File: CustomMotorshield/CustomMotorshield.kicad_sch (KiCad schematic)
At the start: 7 parts, among them J1 Conn_01x20, J2 Conn_01x20

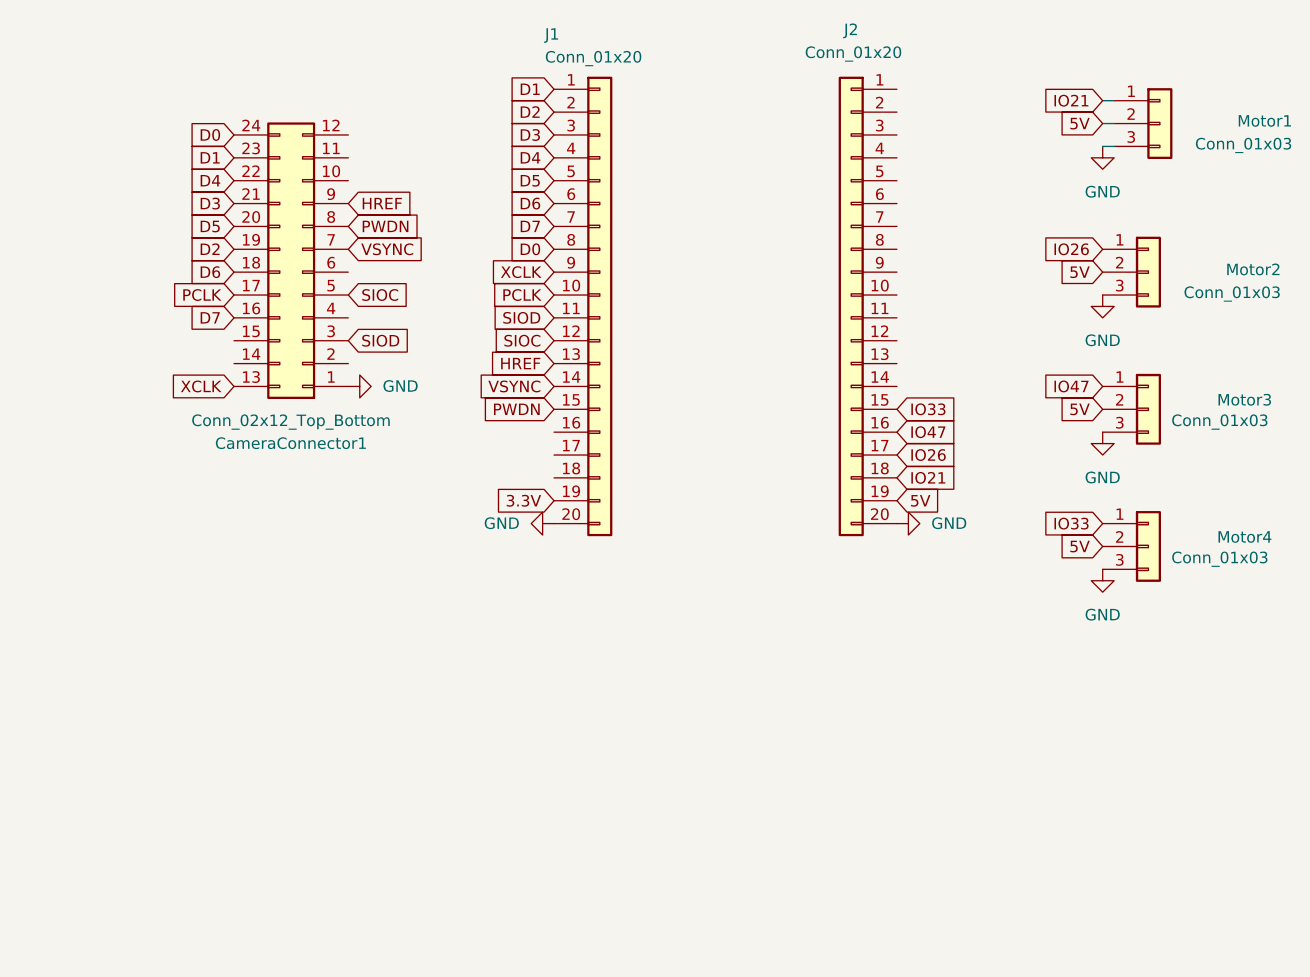
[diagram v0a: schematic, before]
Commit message: Updated PCB !
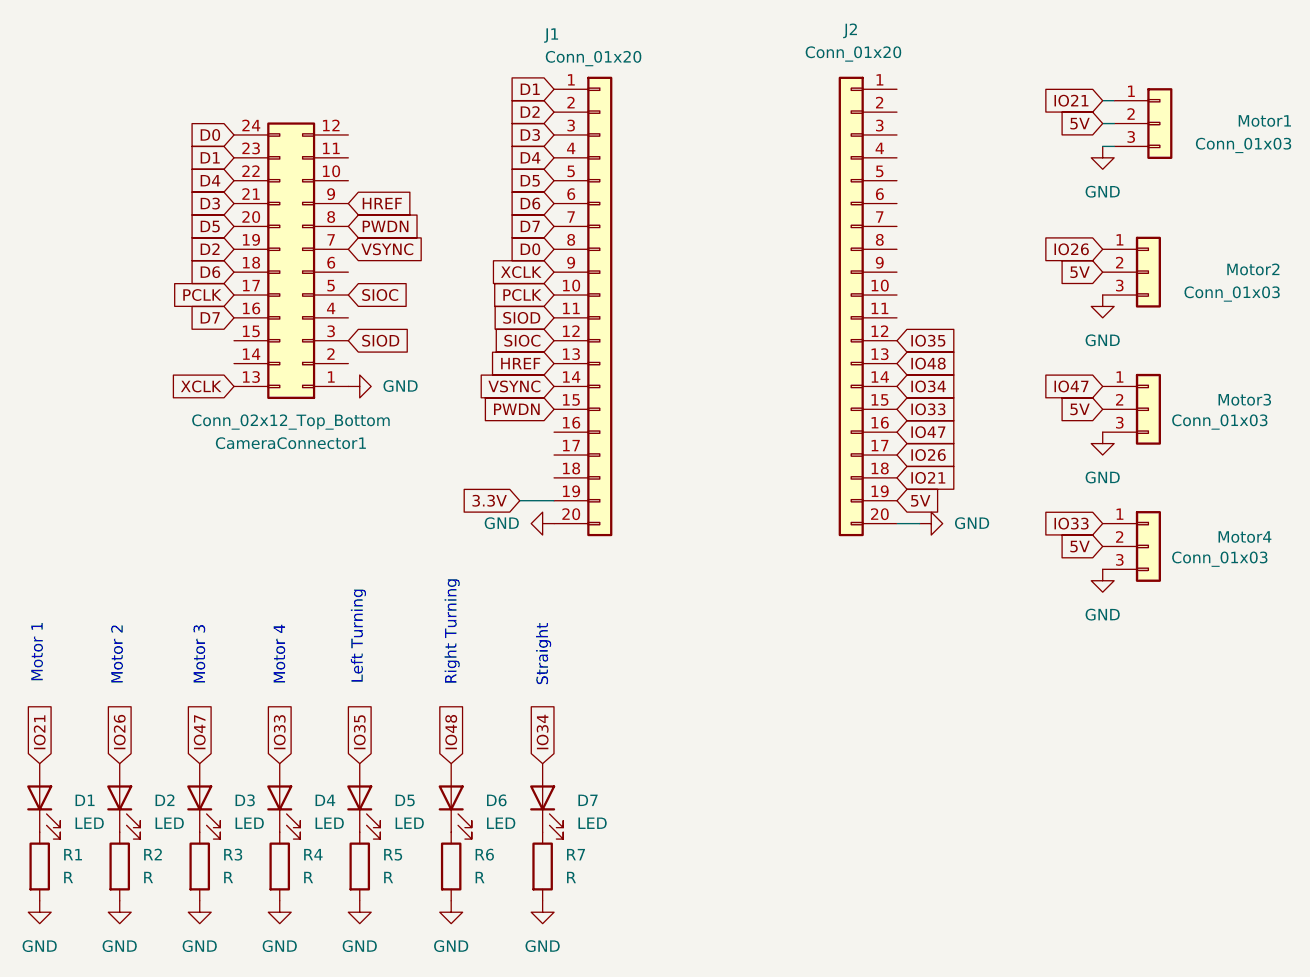
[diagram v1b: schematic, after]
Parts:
- added D1, D2, D3, D4, D5, D6, D7: LED, LED_SMD:LED_2512_6332Metric, symbol Device:LED
- added R1, R2, R3, R4, R5, R6, R7: R, Resistor_SMD:R_1206_3216Metric_Pad1.30x1.75mm_HandSolder, symbol Device:R
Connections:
- net GND: now also R1.2, R2.2, R3.2, R4.2, R5.2, R6.2, R7.2
- net IO21: now also D1.2 (A)
- net IO26: now also D2.2 (A)
- net IO33: now also D4.2 (A)
- net IO47: now also D3.2 (A)
- net IO35: now reaches J2.12 (Pin_12)
- net IO35: now also D5.2 (A)
- net IO48: now reaches J2.13 (Pin_13)
- net IO48: now also D6.2 (A)
- net IO34: now reaches J2.14 (Pin_14)
- net IO34: now also D7.2 (A)
- new net: D2.1 (K), R2.1
- new net: D7.1 (K), R7.1
- new net: D6.1 (K), R6.1
- new net: D4.1 (K), R4.1
- new net: D5.1 (K), R5.1
- new net: D3.1 (K), R3.1
- new net: D1.1 (K), R1.1
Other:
- note added: "Left Turning"
- note added: "Motor 1"
- note added: "Motor 2"
- note added: "Motor 3"
- note added: "Motor 4"
- note added: "Right Turning"
- note added: "Straight"
